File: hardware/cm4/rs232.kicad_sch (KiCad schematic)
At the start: 13 parts, among them J3 D340 PC (4P4C), U3 ADuM5211, U5 MAX3232E

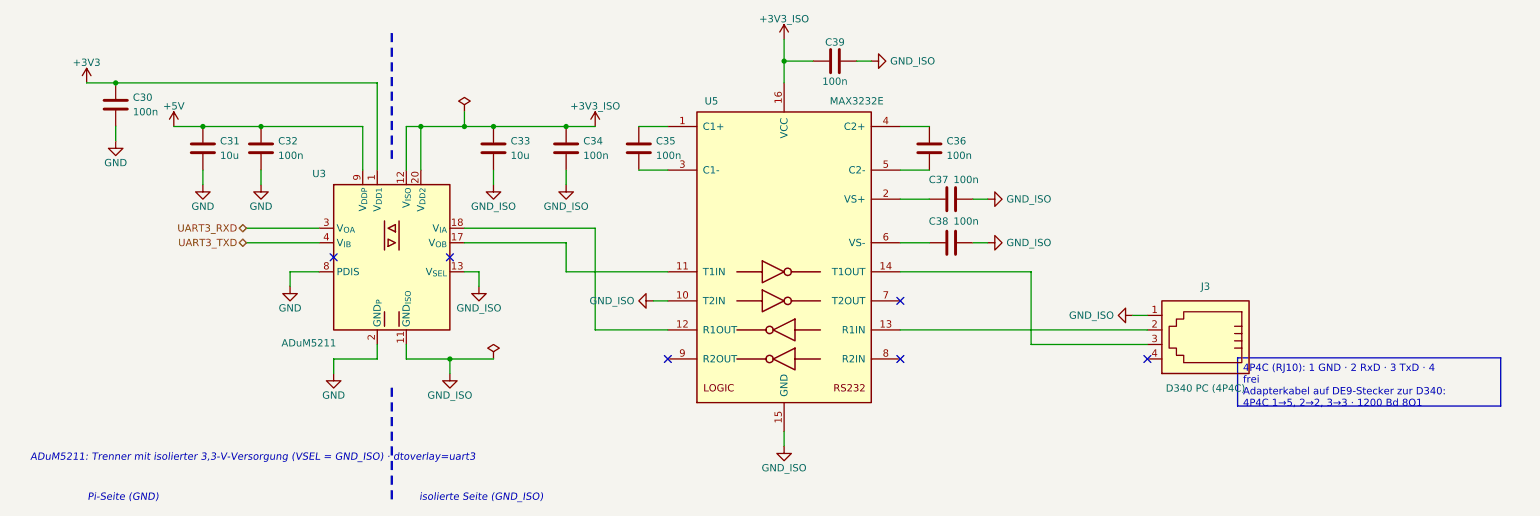
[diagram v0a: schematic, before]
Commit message: CM4-Schaltplan: Handänderungen übernommen (Handlage für 8 Blätter, 2 Texte zurückgeführt); Kastenhöhen aus gemessenen Zeichenbreiten
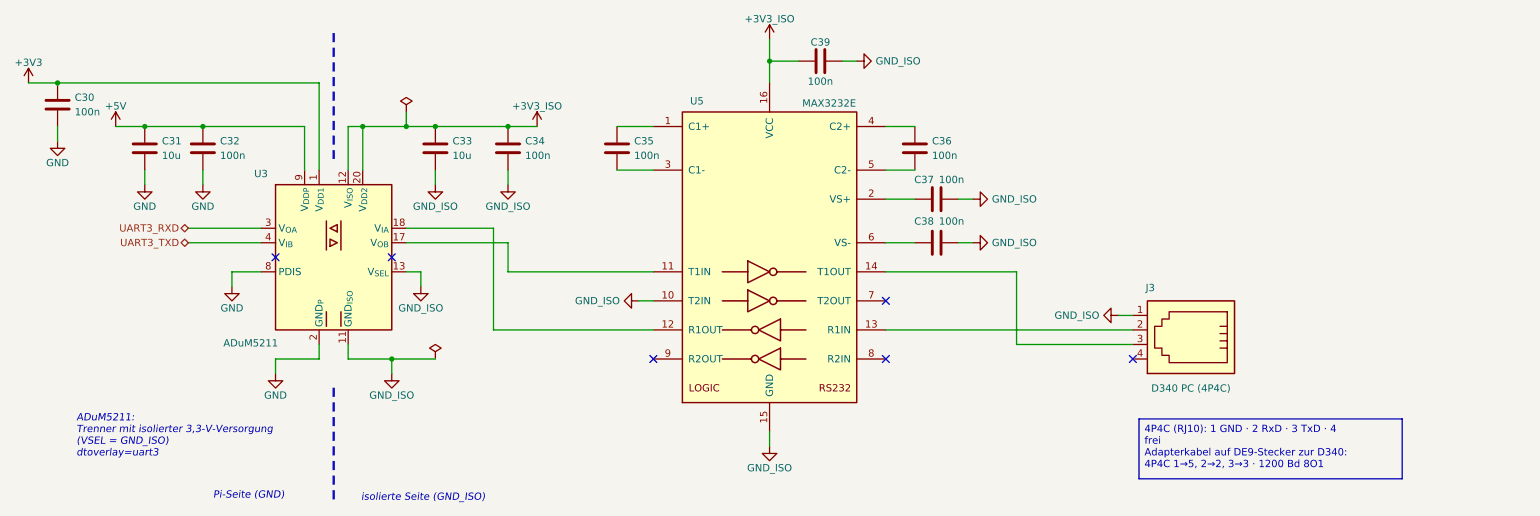
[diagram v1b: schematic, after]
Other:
- note added: "ADuM5211: Trenner mit isolierter 3,3-V-Versorgung (VSEL = GND_ISO) dtoverlay=uart3"
- note removed: "ADuM5211: Trenner mit isolierter 3,3-V-Versorgung (VSEL = GND_ISO) · dtoverlay=uart3"
- moved on the sheet: C30, C31, C32, C33, C34, C35, C36, C37, C38, C39, J3, U3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
